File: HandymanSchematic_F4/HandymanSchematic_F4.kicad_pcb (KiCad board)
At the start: 4 copper layers, 55.6 x 45.5 mm, 76 parts, among them J1 SWD Header, J2 JACKS, J5 ScopeGroundLoop, Q1 BC847, Q2 2N7002, Q3 2N7002, SW1 RST, SW2 BYP, SW302 BOOT, U2 TL074, U3 STM32F411RETx, U4 AMS1117, U5 SSD1306, U6 TL072, Y1 16MHz

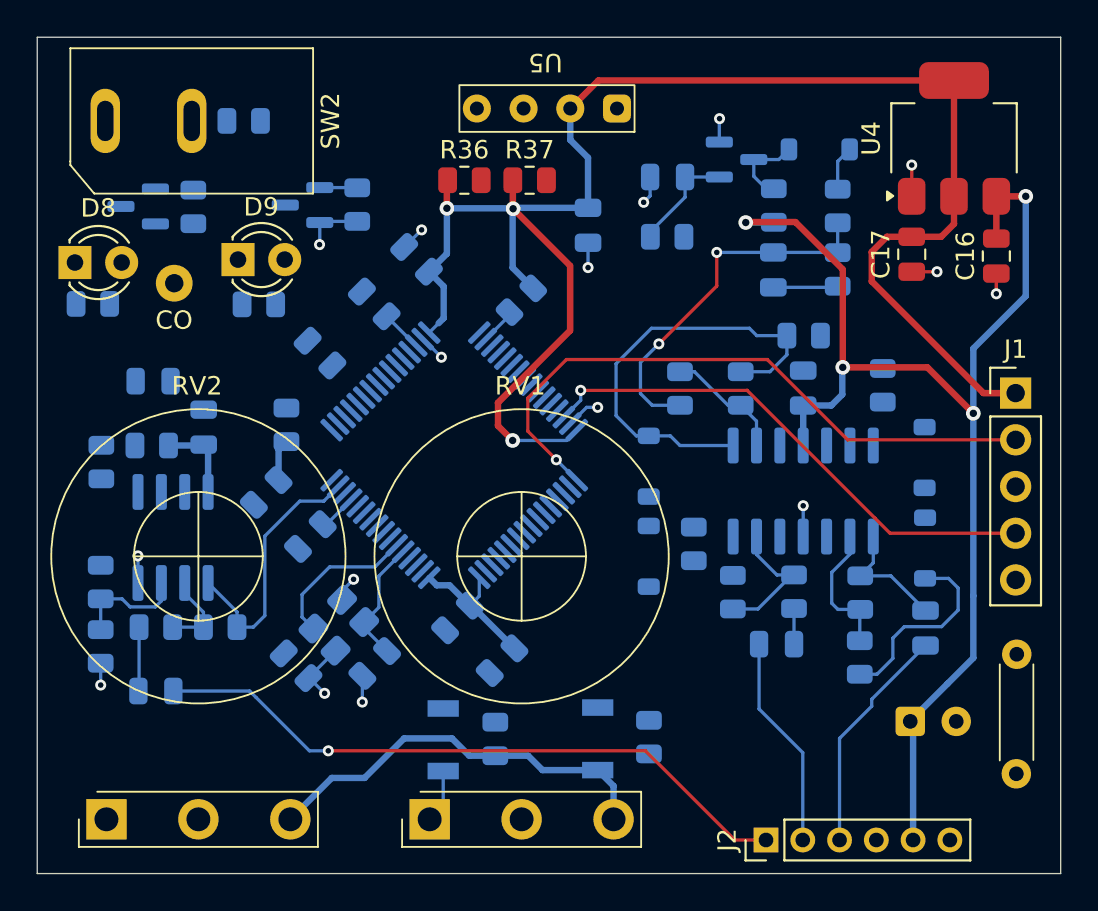
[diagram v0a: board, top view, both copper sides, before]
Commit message: prelim routing
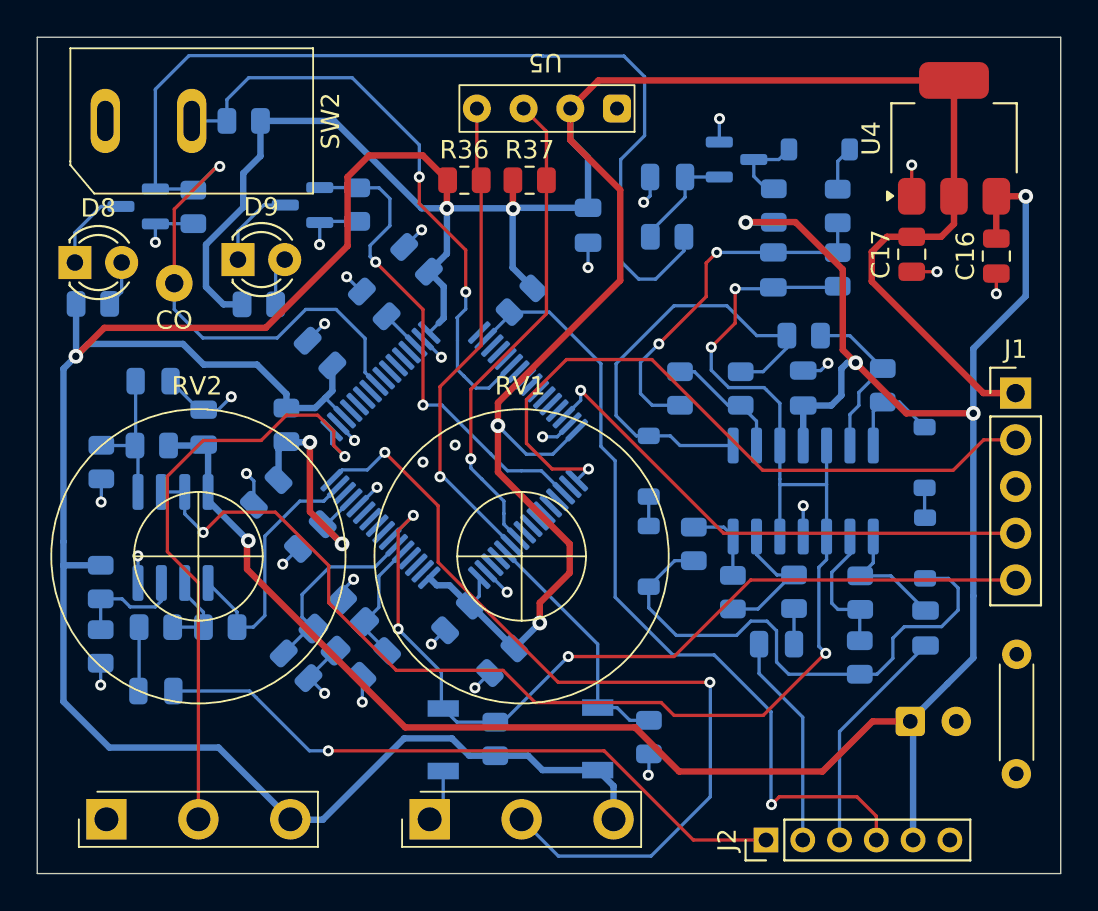
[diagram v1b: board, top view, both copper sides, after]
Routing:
- net +3.3V: track 125.4 -> 257.9 mm, vias 3 -> 5
- net /Analog/VG: track 3.53 -> 81.8 mm, vias 0 -> 4
- net CLOSED_OUT: track 0.00 -> 77.1 mm, vias 0 -> 1
- net NRST: track 0.00 -> 48.3 mm, vias 0 -> 3
- net +9V: track 73.2 -> 120.4 mm, vias 4 -> 5
- net THRESH_IN: track 0.00 -> 46.8 mm, vias 0 -> 2
- net /Digital/TunerModeIn: track 2.00 -> 44.9 mm, vias 0 -> 1
- net RELEASE_IN: track 0.00 -> 33.5 mm, vias 0 -> 1
- net /Digital/GateByp: track 0.00 -> 32.9 mm, vias 0 -> 2
- net /Digital/SCL: track 0.00 -> 26.7 mm, vias 0 -> 1
- net /Digital/SDA: track 0.00 -> 26.5 mm, vias 0 -> 1
- net /Digital/GateLED: track 2.04 -> 26.6 mm, vias 0 -> 2
- net GND: track 29.6 -> 52.9 mm, vias 16 -> 32
- net /Analog/SumPt: track 10.7 -> 29.5 mm
- net /Digital/BOOT0: track 0.00 -> 13.6 mm
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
